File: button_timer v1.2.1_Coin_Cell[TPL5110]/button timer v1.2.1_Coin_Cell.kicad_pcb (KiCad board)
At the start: 2 copper layers, 21 x 47.8 mm, 25 parts, among them J1 Conn_01x05_Female, Q1 TSM2323, SW1 SW_Push, SW2 SW_Push, U1 TPS61097A, U2 TPL5110, X1 ESP-12E

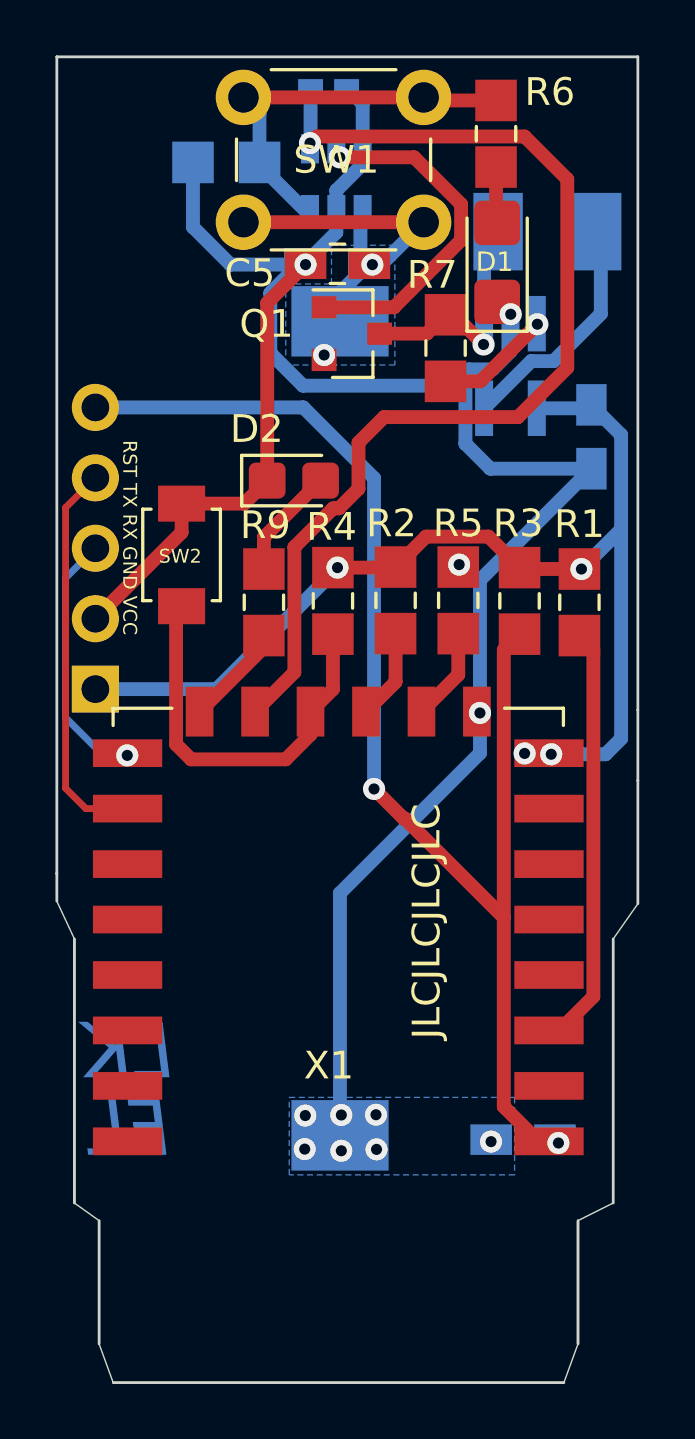
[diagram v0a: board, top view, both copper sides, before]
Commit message: Silkscreen Update
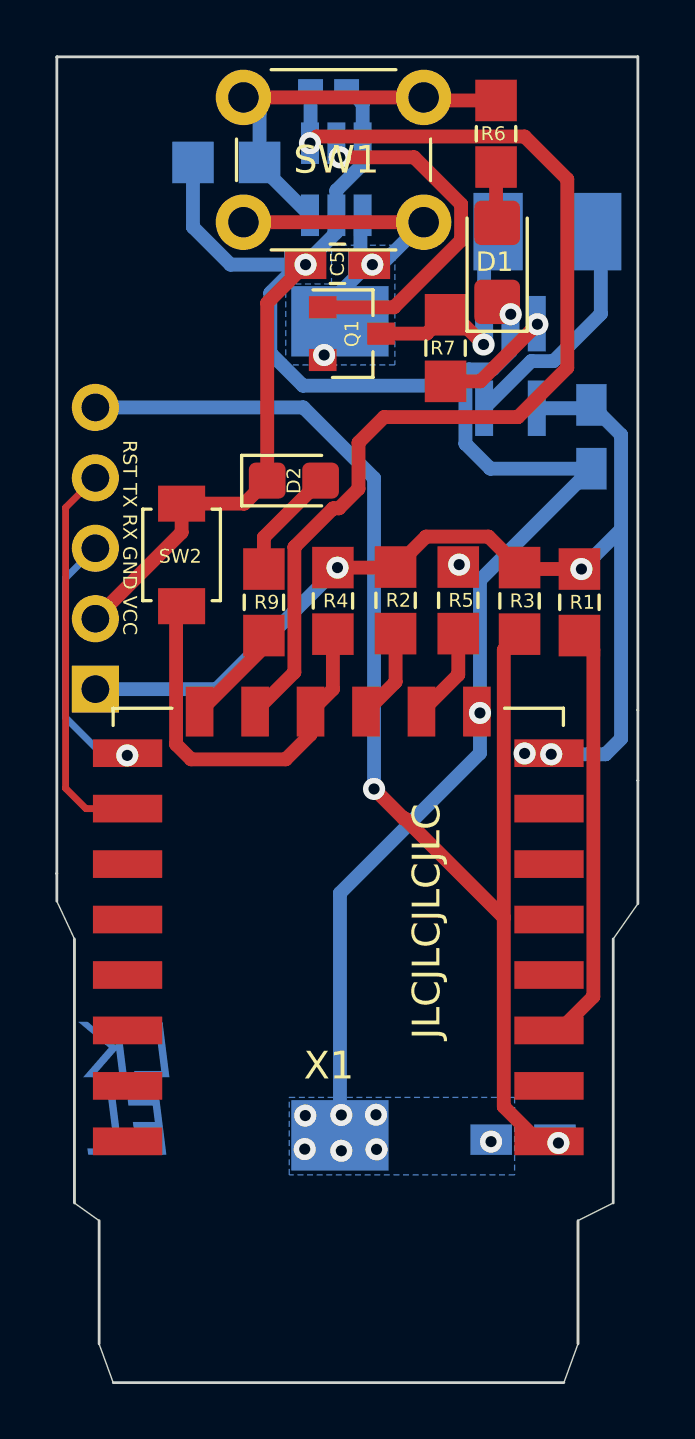
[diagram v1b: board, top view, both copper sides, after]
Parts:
- D2: footprint LED_SMD:LED_0805_2012Metric_Castellated -> handsolder:LED_0805_2012Metric_Castellated_mod
- U2: footprint Package_TO_SOT_SMD:SOT-23-6 -> handsolder:SOT-23-6handsoldering
